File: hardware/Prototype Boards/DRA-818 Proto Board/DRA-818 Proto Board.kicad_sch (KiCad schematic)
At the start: 36 parts, among them Q1 DMN67D8LW-13, Q3 Q_NPN_BCE, SW1 H/L_DIP_SW, U5 LTV-356T

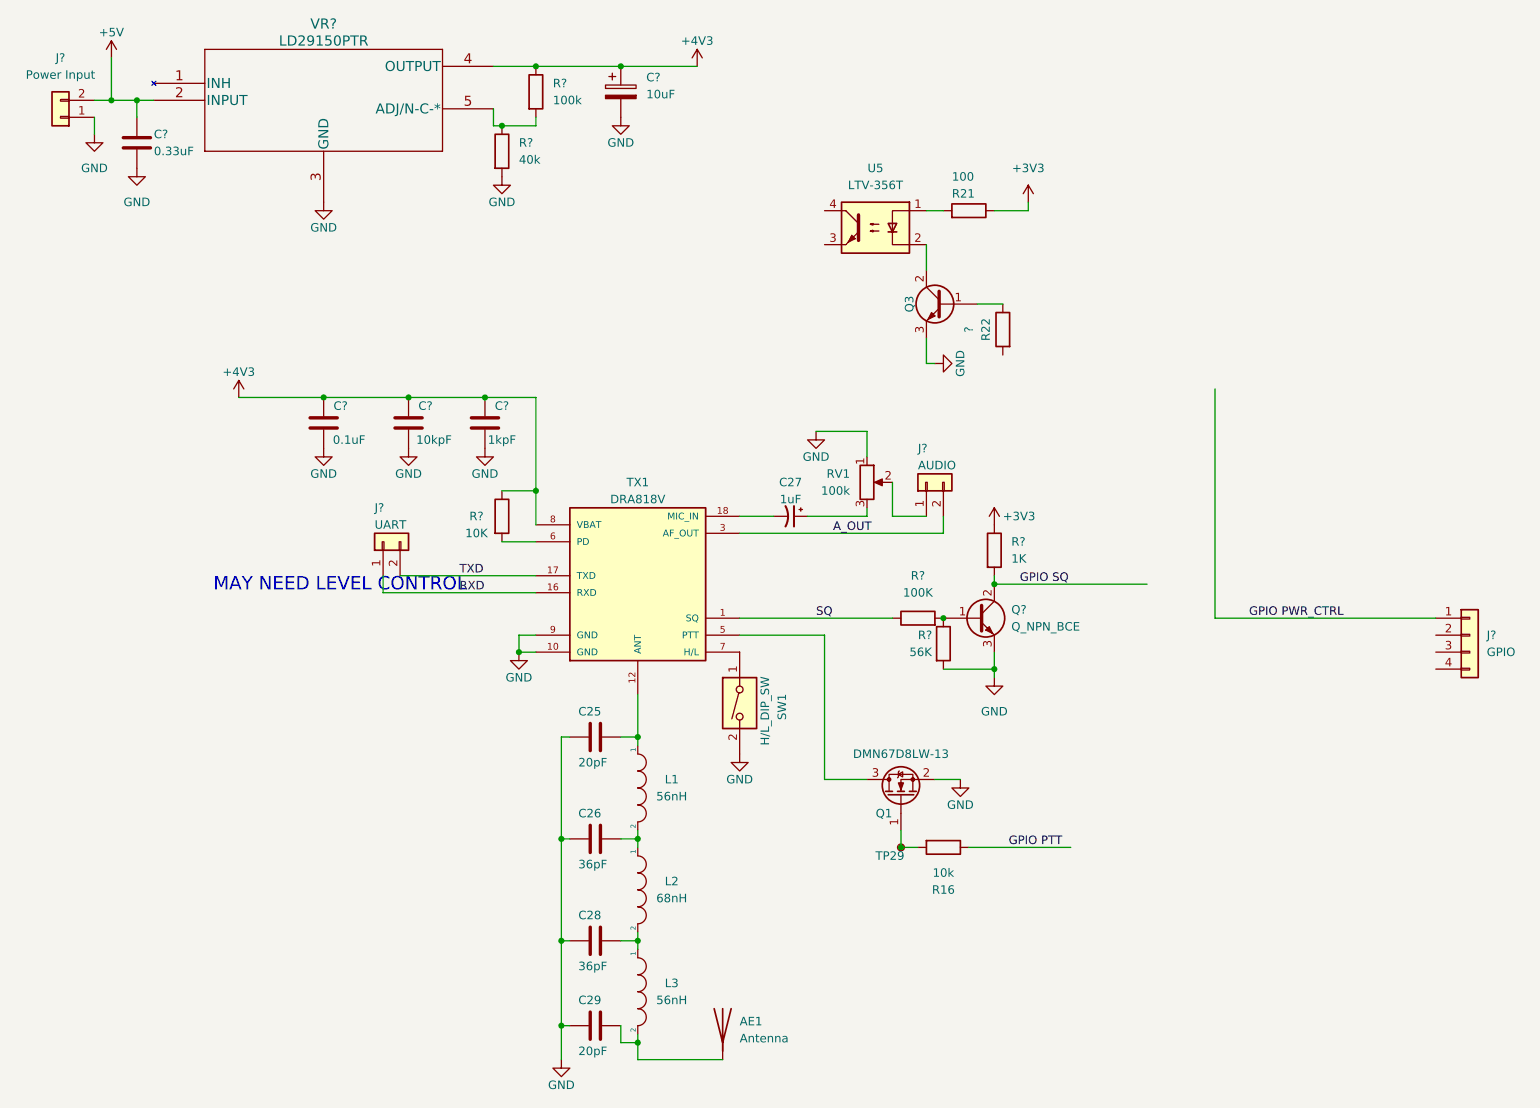
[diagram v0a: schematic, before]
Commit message: GFC RF Proto Board Schematic update
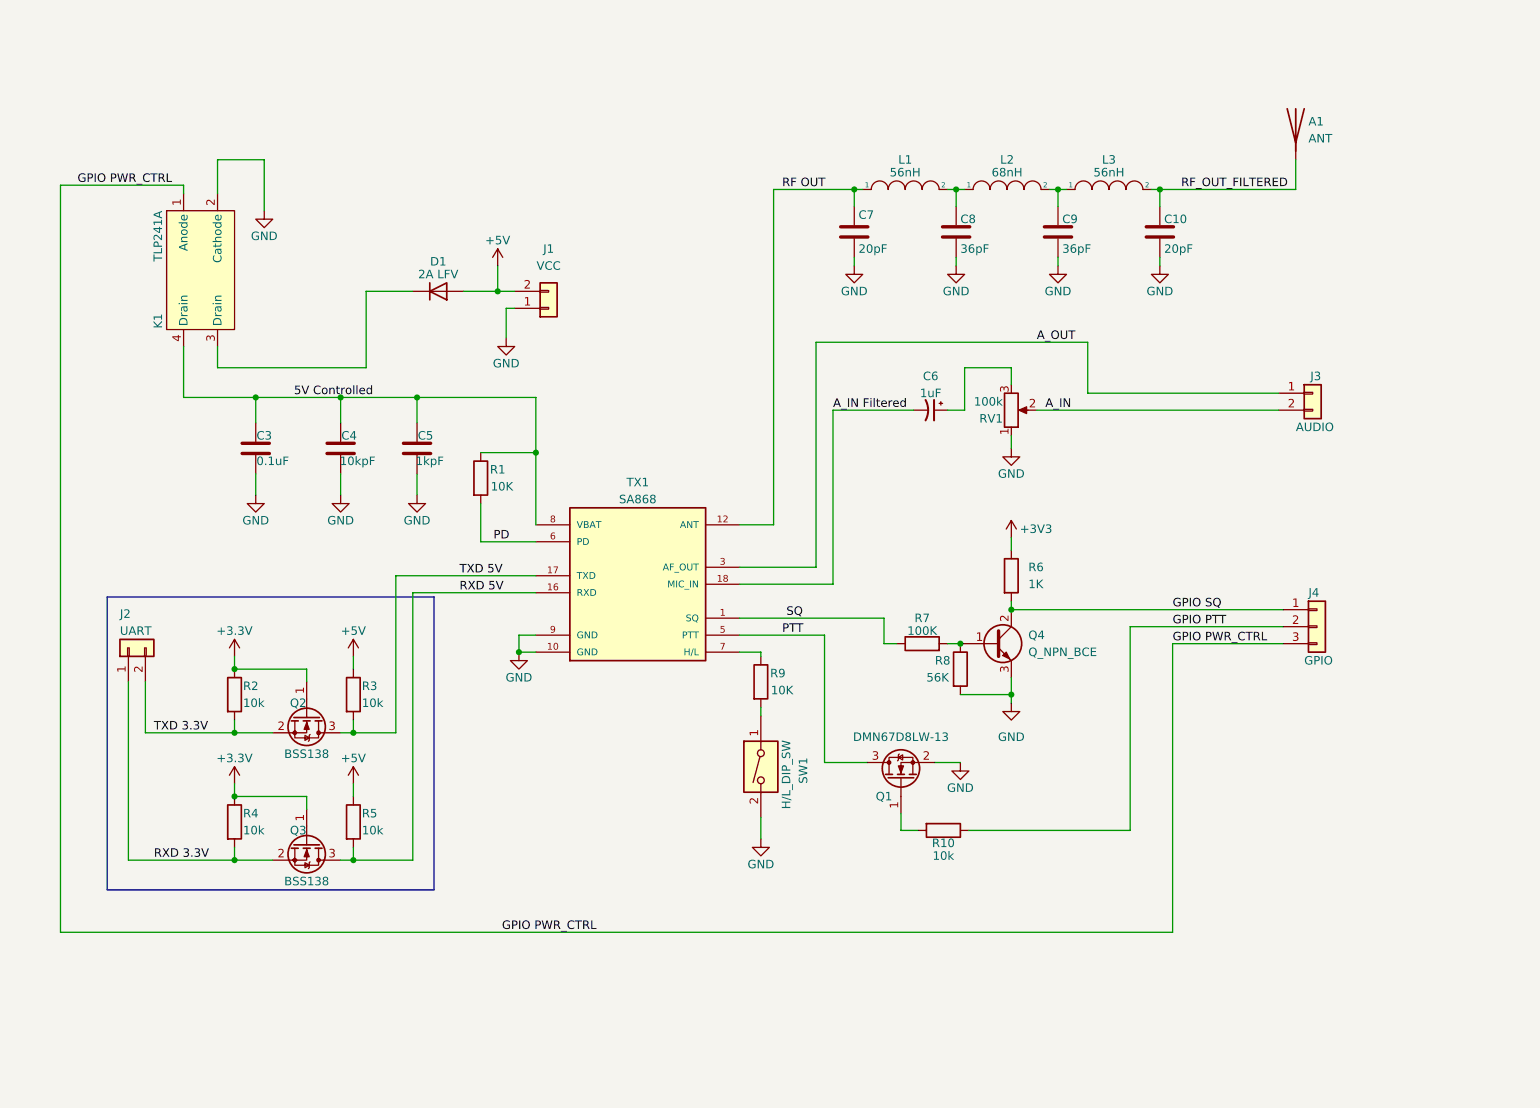
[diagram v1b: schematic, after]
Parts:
- removed AE1: Antenna, footprints:LINX_CONSMA001-G, symbol Device:Antenna
- removed C25, C29: 20pF, Capacitor_SMD:C_0603_1608Metric_Pad1.08x0.95mm_HandSolder, symbol Device:C
- removed C26, C28: 36pF, Capacitor_SMD:C_0603_1608Metric_Pad1.08x0.95mm_HandSolder, symbol Device:C
- removed C?: 0.33uF, symbol Device:C
- removed C?: 10uF, symbol Device:C_Polarized
- removed J?: AUDIO, symbol Connector_Generic:Conn_01x02
- removed J?: UART, symbol Connector_Generic:Conn_01x02
- removed Q3: Q_NPN_BCE, Package_TO_SOT_SMD:SOT-23, symbol Device:Q_NPN_BCE
- removed R21: 100, Resistor_SMD:R_0805_2012Metric_Pad1.20x1.40mm_HandSolder, symbol Device:R
- removed R22: ?, Resistor_SMD:R_0603_1608Metric_Pad0.98x0.95mm_HandSolder, symbol Device:R
- removed R?: 100k, symbol Device:R
- removed R?: 40k, symbol Device:R
- removed TP29: Test Point, TestPoint:TestPoint_Pad_D1.0mm, symbol Connector:TestPoint_Small
- removed U5: LTV-356T, Package_SO:SO-4_4.4x3.6mm_P2.54mm, symbol Isolator:LTV-356T
- removed VR?: LD29150PTR, footprints:LD29150PTR, symbol GFC-Symbols:LD29150PTR
- added A1: ANT, GFC-Footprints:LINX_CONSMA001-G, symbol Device:Antenna
- added C10, C7: 20pF, Capacitor_SMD:C_0603_1608Metric_Pad1.08x0.95mm_HandSolder, symbol Device:C
- added C8, C9: 36pF, Capacitor_SMD:C_0603_1608Metric_Pad1.08x0.95mm_HandSolder, symbol Device:C
- added D1: 2A LFV, Diode_SMD:D_SMA, symbol Device:D
- added J2: UART, Connector_PinHeader_2.54mm:PinHeader_1x02_P2.54mm_Vertical, symbol Connector_Generic:Conn_01x02
- added J3: AUDIO, Connector_PinHeader_2.54mm:PinHeader_1x02_P2.54mm_Vertical, symbol Connector_Generic:Conn_01x02
- added K1: TLP241A, Package_DIP:DIP-4_W8.89mm_SMDSocket_LongPads, symbol GFC-Symbols:TLP241A
- added Q2, Q3: BSS138, Package_TO_SOT_SMD:SOT-23, symbol Transistor_FET:BSS138
- added R2, R3, R4, R5: 10k, Resistor_SMD:R_0603_1608Metric_Pad0.98x0.95mm_HandSolder, symbol Device:R
- added R9: 10K, Resistor_SMD:R_0603_1608Metric_Pad0.98x0.95mm_HandSolder, symbol Device:R
- C3: renamed from C?; Digikey https://www.digikey.com/short/3wn2fdb2 -> -
- C4: renamed from C?; Digikey https://www.digikey.com/short/0b20twhm -> -
- C5: renamed from C?; Digikey https://www.digikey.com/short/wt1rq83j -> -
- C6: renamed from C27; footprint Capacitor_SMD:C_0603_1608Metric_Pad1.08x0.95mm_HandSolder -> Capacitor_SMD:C_0805_2012Metric_Pad1.18x1.45mm_HandSolder; Digikey https://www.digikey.com/short/mb0p55bt -> -
- J1: renamed from J?; value Power Input -> VCC; footprint (none) -> Connector_PinHeader_2.54mm:PinHeader_1x02_P2.54mm_Vertical
- J4: renamed from J?; footprint (none) -> Connector_PinHeader_2.54mm:PinHeader_1x03_P2.54mm_Vertical; symbol Connector_Generic:Conn_01x04 -> Connector_Generic:Conn_01x03
- L1, L3: footprint footprints:IND_AIAC-1812-33NK-T -> GFC-Footprints:IND_AIAC-1812-33NK-T; Digikey https://www.digikey.com/short/9vrrnz3q -> -
- L2: footprint footprints:IND_AIAC-1812-33NK-T -> GFC-Footprints:IND_AIAC-1812-33NK-T; Digikey https://www.digikey.com/short/p9jjjhfr -> -
- Q1: Digikey https://www.digikey.com/short/vpj3wh87 -> -
- Q4: renamed from Q?; Digikey https://www.digikey.com/short/b477vdt4 -> -
- R1: renamed from R?; footprint Resistor_SMD:R_0805_2012Metric_Pad1.20x1.40mm_HandSolder -> Resistor_SMD:R_0603_1608Metric_Pad0.98x0.95mm_HandSolder; Digikey https://www.digikey.com/short/qp0zwmnj -> -
- R10: renamed from R16; footprint Resistor_SMD:R_0805_2012Metric_Pad1.20x1.40mm_HandSolder -> Resistor_SMD:R_0603_1608Metric_Pad0.98x0.95mm_HandSolder; Digikey https://www.digikey.com/short/qp0zwmnj -> -
- R6: renamed from R?; Digikey https://www.digikey.com/short/f10jtr77 -> -
- R7: renamed from R?; Digikey https://www.digikey.com/short/djq9jdpp -> -
- R8: renamed from R?; Digikey https://www.digikey.com/short/bj31bf3h -> -
- RV1: footprint footprints:TRIM_3361P-1-104GLF -> GFC-Footprints:TRIM_3361P-1-104GLF; Digikey https://www.digikey.com/short/vp58mvrf -> -
- SW1: Digikey https://www.digikey.com/short/hh7p03qq -> -
- TX1: value DRA818V -> SA868; footprint footprints:DORJI_DRA818V -> GFC-Footprints:DORJI_DRA818V; symbol GFC-Symbols:DRA818V -> GFC-Symbols:SA868; MANUFACTURER DORJI -> NiceRF
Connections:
- net +5V: now also D1.2 (A), R3.1, R5.1
- net A_OUT: now also J3.1 (Pin_1)
- net GND: now also C10.2, C7.2, C8.2, C9.2, K1.2 (Cathode)
- net GPIO PTT: now also J4.2 (Pin_2)
- net GPIO PWR_CTRL: now also J4.3 (Pin_3), K1.1 (Anode); no longer J4.1 (Pin_1)
- net GPIO SQ: now also J4.1 (Pin_1)
- net at L1.2, L2.1: now also C8.1
- net at L2.2, L3.1: now also C9.1
- net A_IN: now reaches RV1.2
- net A_IN: now also J3.2 (Pin_2)
- net RF_OUT_FILTERED: now reaches L3.2
- net RF_OUT_FILTERED: now also A1.1 (A), C10.1
- net RF OUT: now reaches L1.1, TX1.12 (ANT)
- net RF OUT: now also C7.1
- net PD: now reaches R1.2, TX1.6 (PD)
- net at TX1.7 (H/L): now also R9.1; no longer SW1.1
- net PTT: now reaches Q1.3 (D), TX1.5 (PTT)
- net A_IN Filtered: now reaches C6.2, TX1.18 (MIC_IN)
- net +4V3 renamed 5V Controlled
- net 5V Controlled: now also K1.4 (Drain)
- net RXD renamed RXD 5V
- net RXD 5V: now also Q3.3 (D), R5.2
- net TXD renamed TXD 5V
- net TXD 5V: now also Q2.3 (D), R3.2
- new net: D1.1 (K), K1.3 (Drain)
- new net: R9.2, SW1.1
- new net +3.3V: Q2.1 (G), Q3.1 (G), R2.1, R4.1
- new net RXD 3.3V: J2.1 (Pin_1), Q3.2 (S), R4.2
- new net TXD 3.3V: J2.2 (Pin_2), Q2.2 (S), R2.2
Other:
- note removed: "MAY NEED LEVEL CONTROL"
- moved on the sheet: C3, C4, C5, C6, J1, Q1, Q4, R1, R10, R6, R7, R8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
